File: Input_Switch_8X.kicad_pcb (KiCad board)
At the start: 2 copper layers, 133 x 50 mm, 88 parts, among them J1 Conn_01x02, J10 GND, J2 Conn_01x02, J3 Conn_01x02, J4 Conn_01x02, J5 Conn_01x02, J6 Conn_01x02, J7 Conn_01x02, J8 Conn_01x02, J9 VCC, Q1 AO3400A, Q10 AO3400A, Q11 BC817, Q12 AO3400A, Q13 BC817, Q14 AO3400A, Q15 BC817, Q16 AO3400A, Q2 BC817, Q3 BC817, Q4 AO3400A, Q5 BC817, Q6 AO3400A, Q7 BC817, Q8 AO3400A, Q9 BC817, SW1 SW_Push, SW10 SW_SPST, SW11 SW_Push, SW12 SW_SPST, SW13 SW_Push, SW14 SW_SPST, SW15 SW_Push, SW16 SW_SPST, SW2 SW_SPST, SW3 SW_Push, SW4 SW_SPST, SW5 SW_Push, SW6 SW_SPST, SW7 SW_Push, SW8 SW_SPST, SW9 SW_Push

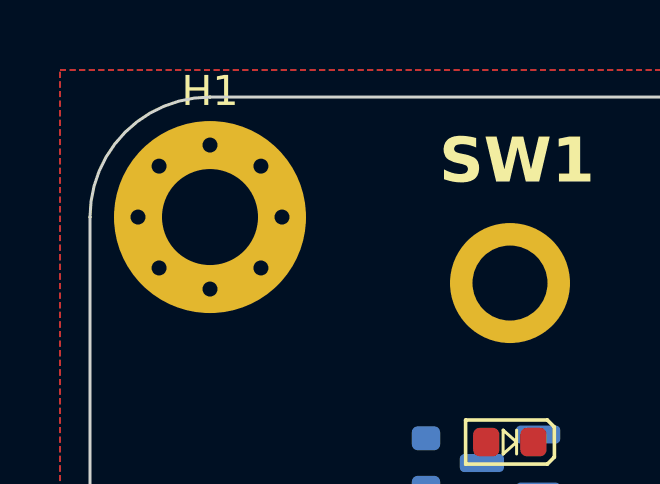
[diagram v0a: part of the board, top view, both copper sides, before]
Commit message: update
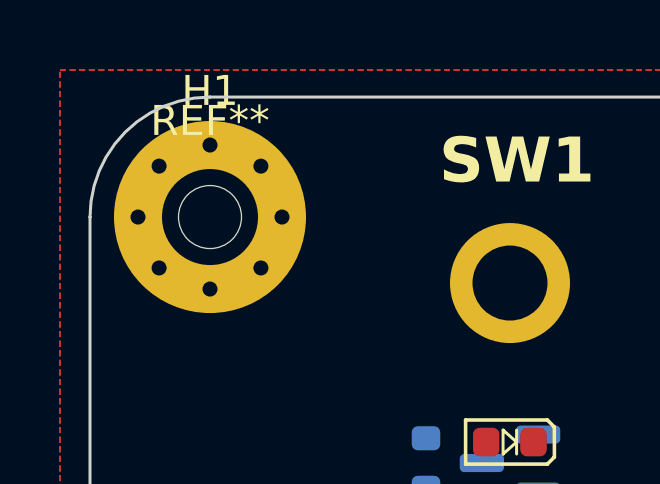
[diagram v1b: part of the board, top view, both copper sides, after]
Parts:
- added REF**: MountingHole_2.1mm, MountingHole:MountingHole_2.1mm, F.Cu at (77.0, 47.9)
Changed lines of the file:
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@@
 			)
 		)
+		(model "${KIPRJMOD}/3D/24.106.STEP"
+			(offset
+				(xyz 0 0 3.81)
+			)
+			(scale
+				(xyz 1 1 1)
+			)
+			(rotate
+				(xyz 0 0 0)
+			)
+		)
 	)
 	(footprint "Library:MountingHole_2.5mm_Pad"
@@
 			)
 		)
+		(model "${KIPRJMOD}/3D/24.106.STEP"
+			(offset
+				(xyz 0 0 3.81)
+			)
+			(scale
+				(xyz 1 1 1)
+			)
+			(rotate
+				(xyz 0 0 0)
+			)
+		)
 	)
 	(footprint "Library:LED_0603_1608Metric"
@@
 			)
 		)
+		(model "${KIPRJMOD}/3D/24.106.STEP"
+			(offset
+				(xyz 0 0 3.81)
+			)
+			(scale
+				(xyz 1 1 1)
+			)
+			(rotate
+				(xyz 0 0 0)
+			)
+		)
 	)
 	(footprint "Library:SW_Toggle_Blue_wSlots_Nut"
@@
 		)
 	)
+	(footprint "MountingHole:MountingHole_2.1mm"
+		(layer "F.Cu")
+		(at 77 47.9)
+		(descr "Mounting Hole 2.1mm, no annular")
+		(tags "mounting hole 2.1mm no annular")
+		(property "Reference" "REF**"
+			(at 0 -3.2 0)
+			(layer "F.SilkS")
+			(effects
+				(font
+					(size 1 1)
+					(thickness 0.15)
+				)
+			)
+		)
+		(property "Value" "MountingHole_2.1mm"
+			(at 0 3.2 0)
+			(layer "F.Fab")
+			(effects
+				(font
+					(size 1 1)
+					(thickness 0.15)
+				)
+			)
+		)
+		(property "Footprint" "MountingHole:MountingHole_2.1mm"
+			(at 0 0 0)
+			(unlocked yes)
+			(layer "F.Fab")
+			(hide yes)
+			(effects
+				(font
+					(size 1.27 1.27)
+				)
+			)
+		)
+		(property "Datasheet" ""
+			(at 0 0 0)
+			(unlocked yes)
+			(layer "F.Fab")
+			(hide yes)
+			(effects
+				(font
+					(size 1.27 1.27)
+				)
+			)
+		)
+		(property "Description" ""
+			(at 0 0 0)
+			(unlocked yes)
+			(layer "F.Fab")
+			(hide yes)
+			(effects
+				(font
+					(size 1.27 1.27)
+				)
+			)
+		)
+		(attr exclude_from_pos_files exclude_from_bom)
+		(fp_circle
+			(center 0 0)
+			(end 2.1 0)
+			(stroke
+				(width 0.15)
+				(type solid)
+			)
+			(fill none)
+			(layer "Cmts.User")
+		)
+		(fp_circle
+			(center 0 0)
+			(end 2.35 0)
+			(stroke
+				(width 0.05)
+				(type solid)
+			)
+			(fill none)
+			(layer "F.CrtYd")
+		)
+		(fp_text user "${REFERENCE}"
+			(at 0 0 0)
+			(layer "F.Fab")
+			(effects
+				(font
+					(size 1 1)
+					(thickness 0.15)
+				)
+			)
+		)
+		(pad "" np_thru_hole circle
+			(at 0 0)
+			(size 2.1 2.1)
+			(drill 2.1)
+			(layers "*.Cu" "*.Mask")
+		)
+		(model "${KIPRJMOD}/3D/Input_Switch_8X.wrl"
+			(offset
+				(xyz -77 48.5 -12.5)
+			)
+			(scale
+				(xyz 1 1 1)
+			)
+			(rotate
+				(xyz 0 0 0)
+			)
+		)
+	)
 	(footprint "Library:MountingHole_2.5mm_Pad"
 		(layer "F.Cu")
@@
 			)
 		)
+		(model "${KIPRJMOD}/3D/24.106.STEP"
+			(offset
+				(xyz 0 0 3.81)
+			)
+			(scale
+				(xyz 1 1 1)
+			)
+			(rotate
+				(xyz 0 0 0)
+			)
+		)
 	)
 	(footprint "Library:LED_0603_1608Metric"
@@
 			)
 		)
+		(model "${KIPRJMOD}/3D/24.106.STEP"
+			(offset
+				(xyz 0 0 3.81)
+			)
+			(scale
+				(xyz 1 1 1)
+			)
+			(rotate
+				(xyz 0 0 0)
+			)
+		)
 	)
 	(footprint "Library:SW_Toggle_Blue_wSlots_Nut"
@@
 			)
 		)
+		(model "${KIPRJMOD}/3D/24.106.STEP"
+			(offset
+				(xyz 0 0 3.81)
+			)
+			(scale
+				(xyz 1 1 1)
+			)
+			(rotate
+				(xyz 0 0 0)
+			)
+		)
 	)
 	(footprint "Library:SW_Toggle_Blue_wSlots_Nut"
@@
 			)
 		)
+		(model "${KIPRJMOD}/3D/24.106.STEP"
+			(offset
+				(xyz 0 0 3.81)
+			)
+			(scale
+				(xyz 1 1 1)
+			)
+			(rotate
+				(xyz 0 0 0)
+			)
+		)
 	)
 	(footprint "Library:LED_0603_1608Metric"
@@
 			)
 		)
+		(model "${KIPRJMOD}/3D/24.106.STEP"
+			(offset
+				(xyz 0 0 3.81)
+			)
+			(scale
+				(xyz 1 1 1)
+			)
+			(rotate
+				(xyz 0 0 0)
+			)
+		)
